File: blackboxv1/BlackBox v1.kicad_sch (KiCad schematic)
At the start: 21 parts, among them J1 Conn_01x04_Socket, J2 USB_C_Receptacle_USB2.0_14P, J3 Conn_01x05_Socket, U1 STM32G0B1CBTx, U2 W25N01GVZEIG_TR, U3 TPS2116DRL

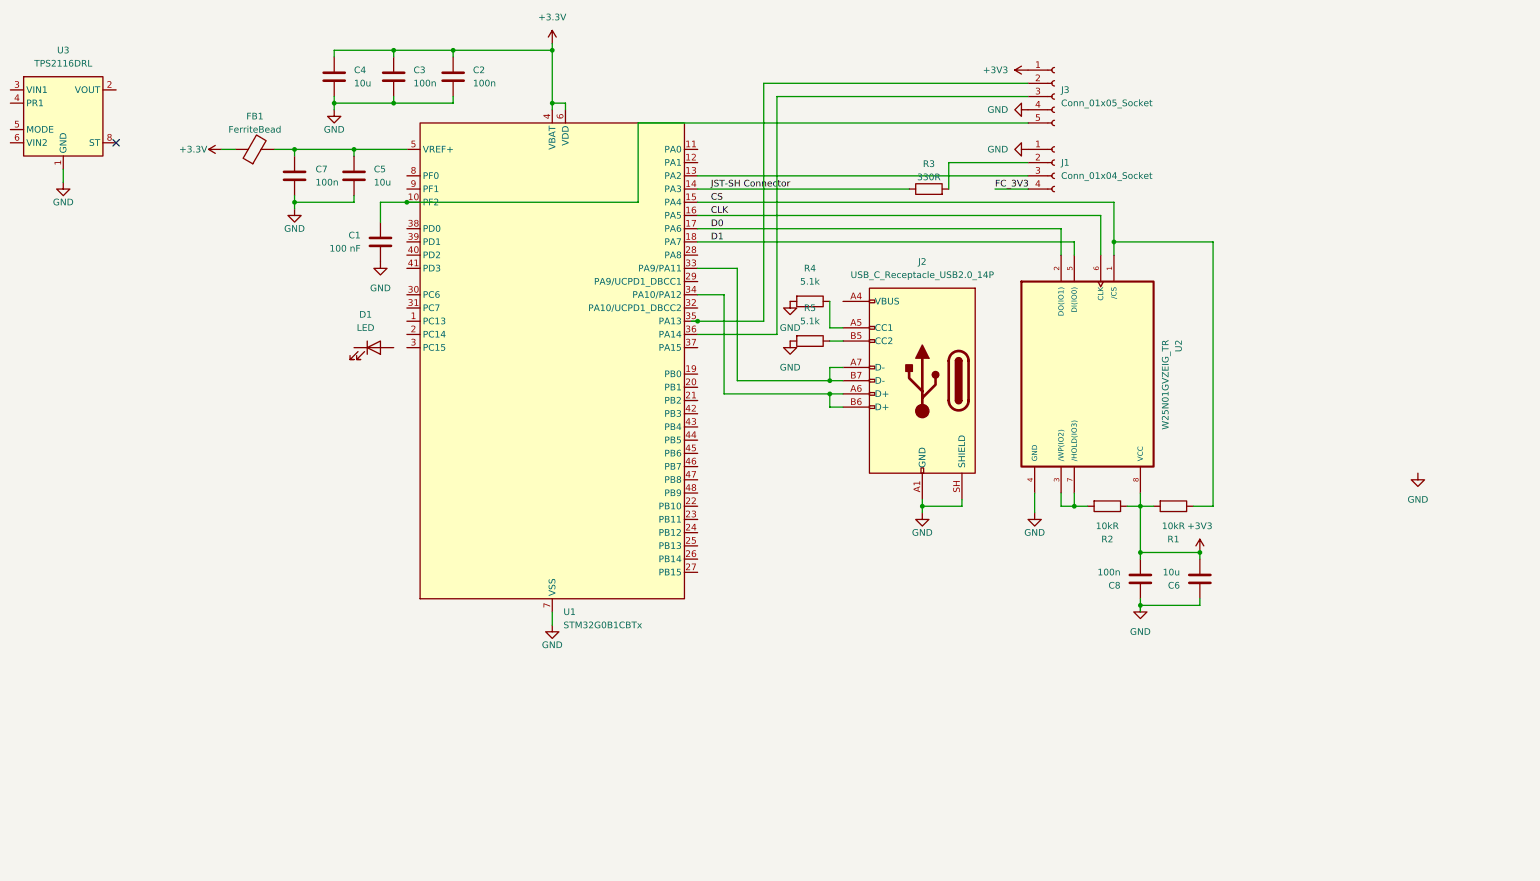
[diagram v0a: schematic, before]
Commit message: Finished Blackbox?
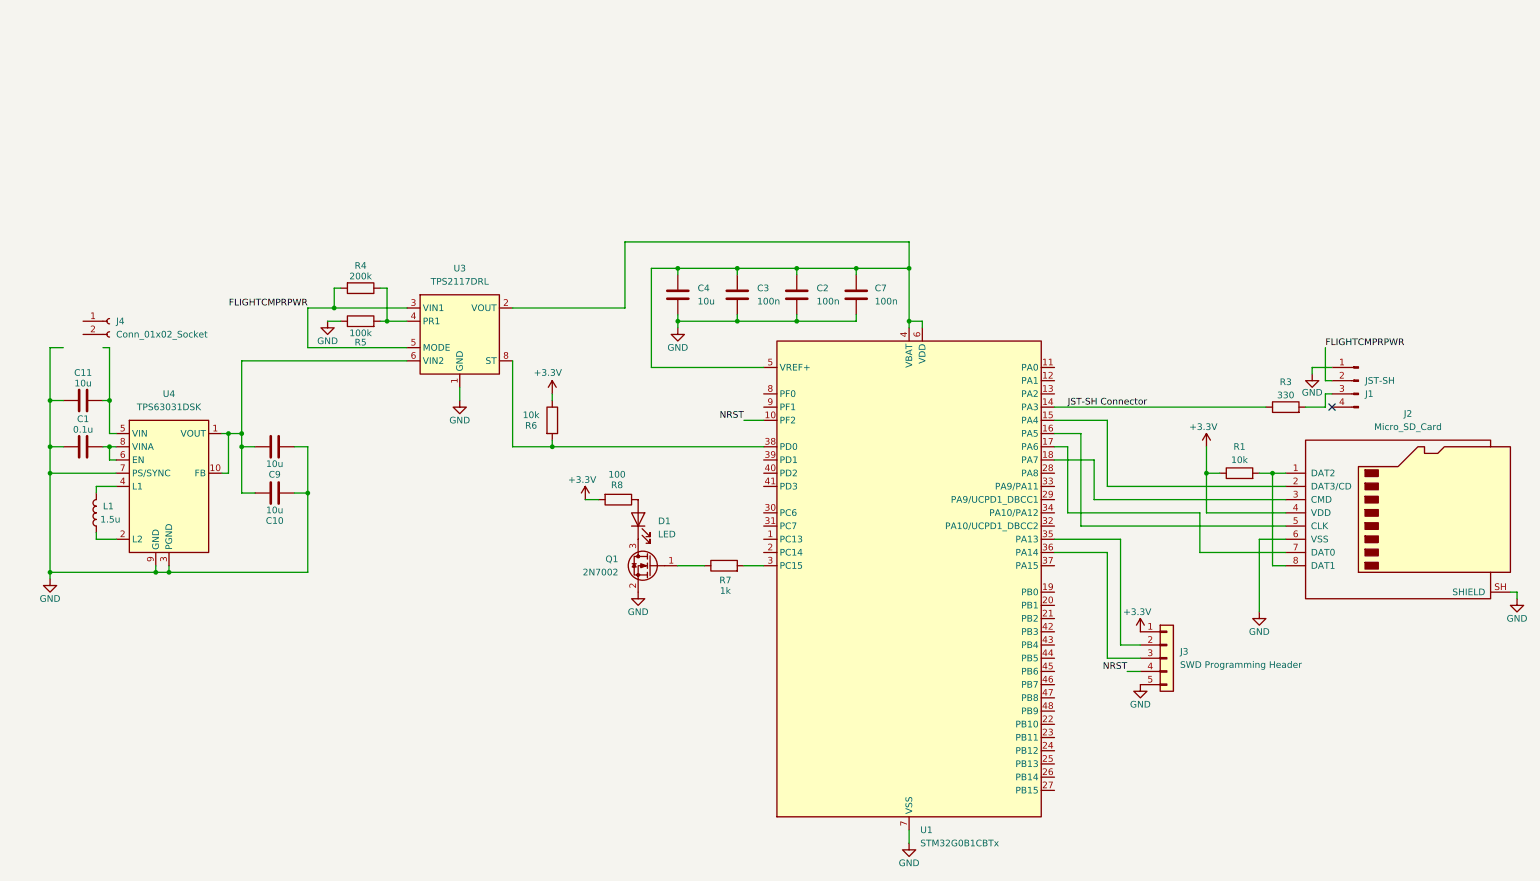
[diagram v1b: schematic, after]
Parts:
- removed C5, C6: 10u, Package_QFP:LQFP-48_7x7mm_P0.5mm, symbol Device:C
- removed C8: 100n, Package_QFP:LQFP-48_7x7mm_P0.5mm, symbol Device:C
- removed FB1: FerriteBead, symbol Device:FerriteBead
- removed J1: Conn_01x04_Socket, symbol Connector:Conn_01x04_Socket
- removed J2: USB_C_Receptacle_USB2.0_14P, symbol Connector:USB_C_Receptacle_USB2.0_14P
- removed J3: Conn_01x05_Socket, symbol Connector:Conn_01x05_Socket
- removed R2: 10kR, symbol Device:R
- removed U2: W25N01GVZEIG_TR, W25N01GVZEIG_TR:SON127P800X600X80-9N, symbol W25N01GVZEIG_TR:W25N01GVZEIG_TR
- added C10, C11, C9: 10u, symbol Device:C
- added J1: JST-SH, OptoDevice:Osram_SMD-SmartDIL, symbol Connector:Conn_01x04_Pin
- added J2: Micro_SD_Card, Connector_Card:microSD_HC_Molex_47219-2001, symbol Connector:Micro_SD_Card
- added J3: SWD Programming Header, symbol Connector_Generic:Conn_01x05
- added J4: Conn_01x02_Socket, Package_SO:SOIC-8_3.9x4.9mm_P1.27mm, symbol Connector:Conn_01x02_Socket
- added L1: 1.5u, Package_SON:WSON-10-1EP_2.5x2.5mm_P0.5mm_EP1.2x2mm, symbol Device:L
- added Q1: 2N7002, Package_TO_SOT_SMD:SOT-23, symbol Transistor_FET:2N7002
- added R6: 10k, symbol Device:R
- added R7: 1k, symbol Device:R
- added R8: 100, symbol Device:R
- added U4: TPS63031DSK, Package_SON:WSON-10-1EP_2.5x2.5mm_P0.5mm_EP1.2x2mm, symbol Regulator_Switching:TPS63031DSK
- C1: value 100 nF -> 0.1u
- R1: value 10kR -> 10k
- R3: value 330R -> 330
- R4: value 5.1k -> 200k; footprint Package_QFP:PQFP-160_28x28mm_P0.65mm -> (none)
- R5: value 5.1k -> 100k; footprint Package_QFP:PQFP-160_28x28mm_P0.65mm -> (none)
- U3: value TPS2116DRL -> TPS2117DRL
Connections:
- net +3.3V: now also R1.1, J2.4 (VDD), J3.1 (Pin_1), R6.1, R8.2; no longer C2.2, C3.2, C4.2, U1.4 (VBAT), U1.6 (VDD)
- net GND: now also C1.1, R5.1, C10.1, C11.1, C9.1, J1.1 (Pin_1), J2.6 (VSS), J2.SH (SHIELD), J3.5 (Pin_5), Q1.2 (S), U4.11 (PGND), U4.3 (PGND), U4.7 (PS/SYNC), U4.9 (GND); no longer C1.2, R4.2, R5.2
- net at R4.1: now also R5.2, U3.4 (PR1)
- net NRST: now reaches U1.10 (PF2)
- net NRST: now also J3.4 (Pin_4); no longer C1.1
- net at U3.2 (VOUT), U3.7 (VOUT): now also C2.2, C3.2, C4.2, C7.1, U1.4 (VBAT), U1.5 (VREF+), U1.6 (VDD)
- net FLIGHTCMPRPWR: now reaches U3.3 (VIN1)
- net FLIGHTCMPRPWR: now also R4.2, U3.5 (MODE), J1.2 (Pin_2)
- net at U3.6 (VIN2): now also C10.2, C9.2, U4.1 (VOUT), U4.10 (FB)
- net at U3.8 (ST): now also U1.38 (PD0), R6.2
- net at R3.2: now also J1.3 (Pin_3)
- net at U1.3 (PC15): now also R7.2
- net at U1.35 (PA13): now also J3.2 (Pin_2)
- net at U1.36 (PA14): now also J3.3 (Pin_3)
- net at D1.1 (K): now also Q1.3 (D)
- net at D1.2 (A): now also R8.1
- net +3V3: no longer names the net of R1.2
- net +3V3: now also J2.1 (DAT2), J2.8 (DAT1)
- net CLK: no longer names the net of U1.16 (PA5)
- net CLK: now also J2.5 (CLK)
- net CS: no longer names the net of U1.15 (PA4)
- net CS: now also J2.2 (DAT3/CD); no longer R1.1
- net D0: no longer names the net of U1.17 (PA6)
- net D0: now also J2.7 (DAT0)
- net D1: no longer names the net of U1.18 (PA7)
- net D1: now also J2.3 (CMD)
- new net: L1.1, U4.2 (L2)
- new net: L1.2, U4.4 (L1)
- new net: C11.2, U4.5 (VIN)
- new net: C1.2, U4.6 (EN), U4.8 (VINA)
- new net: Q1.1 (G), R7.1
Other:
- moved on the sheet: C2, C3, C4, C7, D1, R3, U1, U3
